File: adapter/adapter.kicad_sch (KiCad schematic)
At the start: 28 parts, among them J1 Serial, J10 Ribbon, J11 SPI user, J12 SPI user, J2 Serial, J3 RGB, J4 RGB, J5 Trackball, J6 Ribbon, J7 Trackball, J8 Ribbon, J9 Ribbon, SW1 USER, SW2 USER, U1 STM32F401 / STM32F411 Blackpi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, U2 STM32F401 / STM32F411 Blackpi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

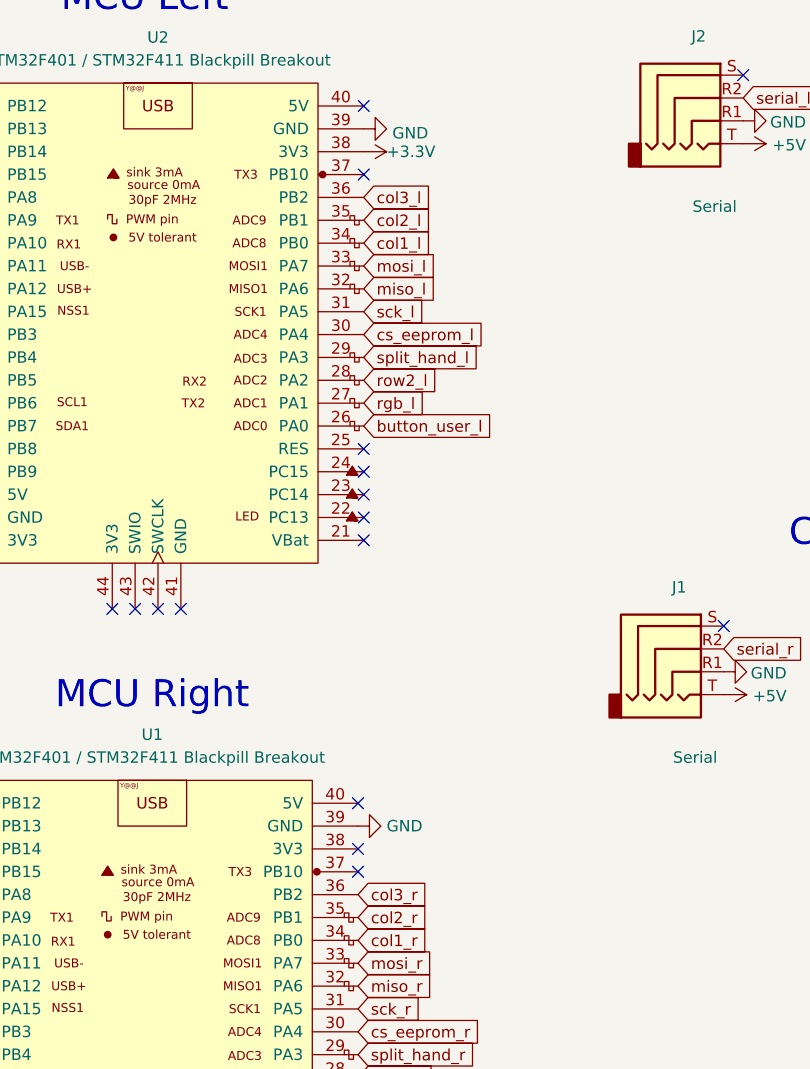
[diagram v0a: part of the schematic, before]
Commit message: Bugfix release 1.1
PB2 has a pulldown on the WeACT board to ensure BOOT1
is low during boot up. Otherwise jumping into the bootloader
is not ensured. So COL3 is moved from PB2 to PB10 as the pull
down prevents this pin from beeing used for matrix scanning.
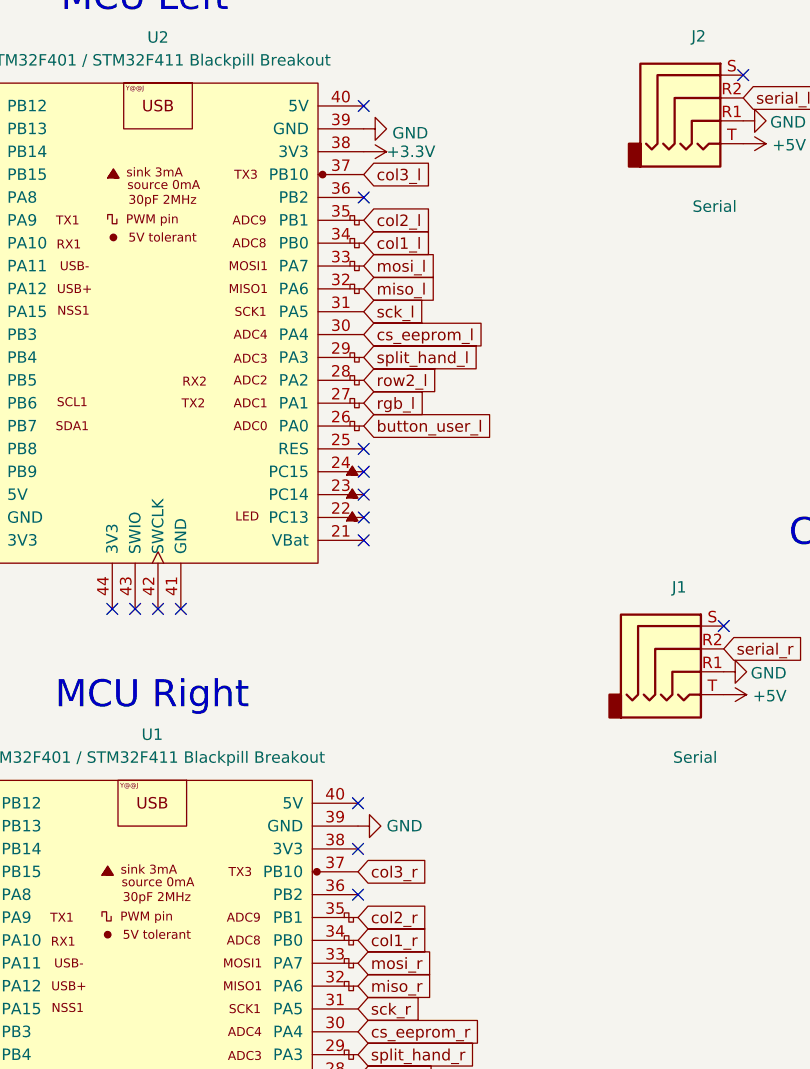
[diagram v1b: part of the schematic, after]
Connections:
- net col3_l: now also U2.37 (PB10); no longer U2.36 (PB2)
- net col3_r: now also U1.37 (PB10); no longer U1.36 (PB2)
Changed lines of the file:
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@@
   (no_connect (at 135.255 168.275))
   (no_connect (at 117.475 112.395))
-  (no_connect (at 163.195 120.015))
   (no_connect (at 118.11 34.925))
+  (no_connect (at 163.195 122.555))
   (no_connect (at 117.475 114.935))
   (no_connect (at 163.195 158.115))
@@
   (no_connect (at 205.994 31.496))
   (no_connect (at 163.83 34.925))
+  (no_connect (at 163.83 45.085))
   (no_connect (at 118.11 37.465))
-  (no_connect (at 163.83 42.545))
   (no_connect (at 163.195 153.035))
   (no_connect (at 118.11 52.705))
@@
     )
   )
-  (global_label "col3_r" (shape input) (at 163.195 122.555 0)
-    (effects (font (size 1.27 1.27)) (justify left))
-    (property "Intersheet References" "${INTERSHEET_REFS}" (id 0) (at 192.405 161.925 0)
+  (global_label "col3_r" (shape input) (at 163.195 120.015 0)
+    (effects (font (size 1.27 1.27)) (justify left))
+    (property "Intersheet References" "${INTERSHEET_REFS}" (id 0) (at 192.405 159.385 0)
       (effects (font (size 1.27 1.27)) hide)
     )
@@
     )
   )
-  (global_label "col3_l" (shape input) (at 163.83 45.085 0)
-    (effects (font (size 1.27 1.27)) (justify left))
-    (property "Intersheet References" "${INTERSHEET_REFS}" (id 0) (at 193.04 84.455 0)
-      (effects (font (size 1.27 1.27)) hide)
-    )
+  (global_label "col3_l" (shape input) (at 163.83 42.545 0)
+    (effects (font (size 1.27 1.27)) (justify left))
+    (property "Intersheet References" "${INTERSHEET_REFS}" (id 0) (at 193.04 81.915 0)
+      (effects (font (size 1.27 1.27)) hide)
+    )

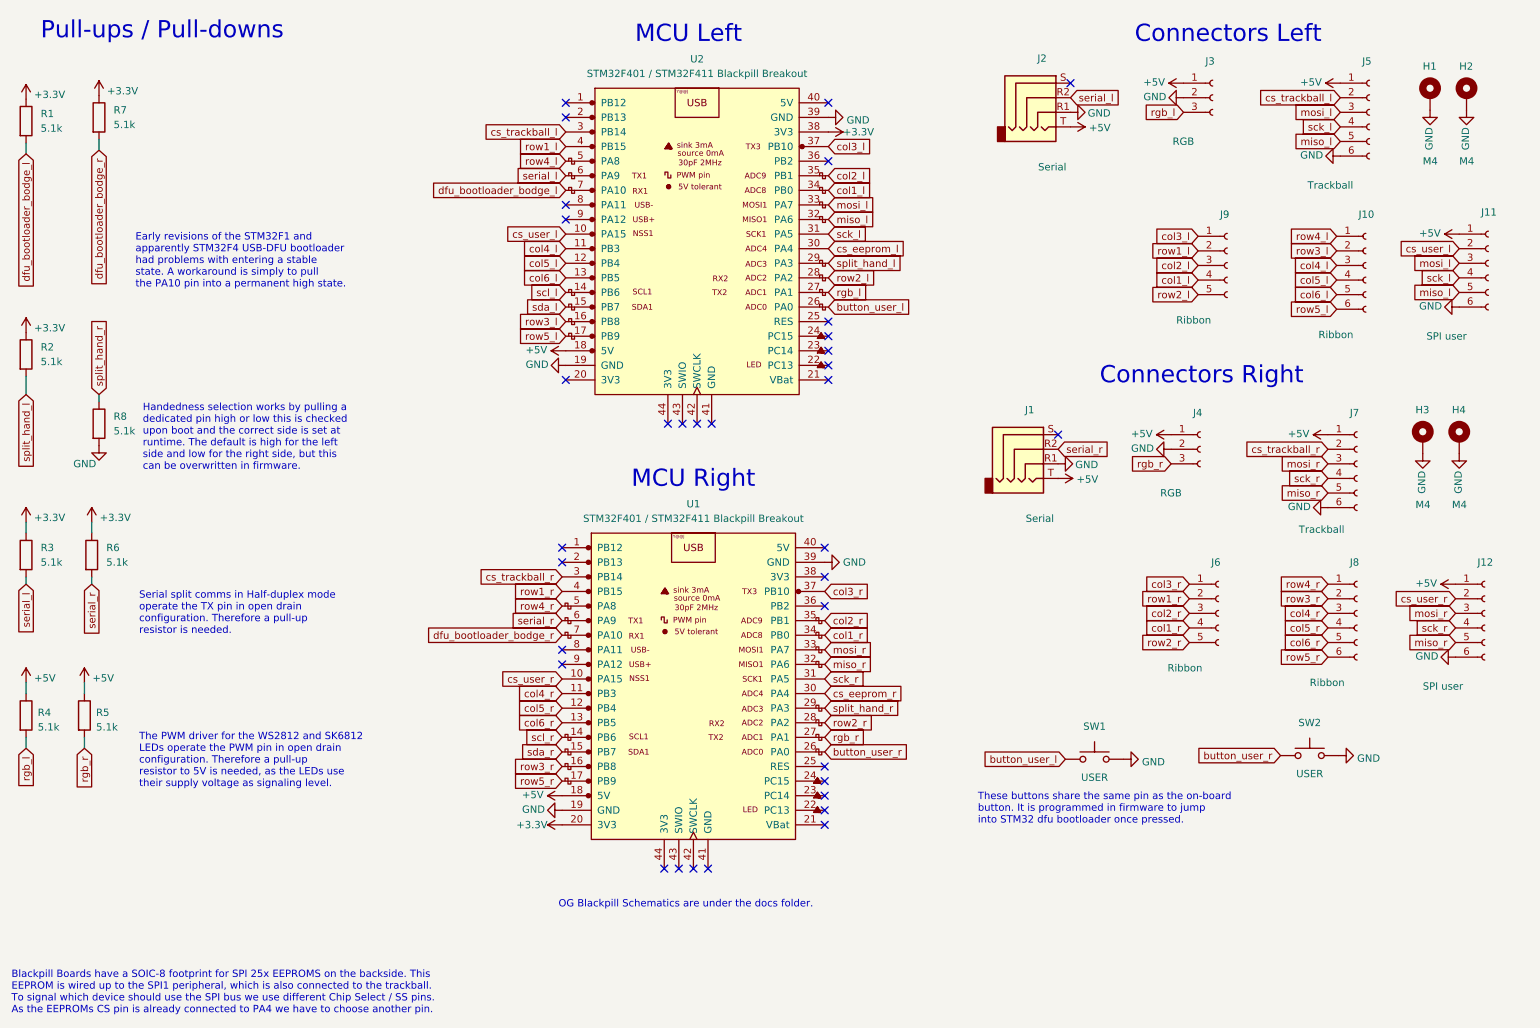
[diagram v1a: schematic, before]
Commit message: Remove SPI user, add breakouts for audio and row 6
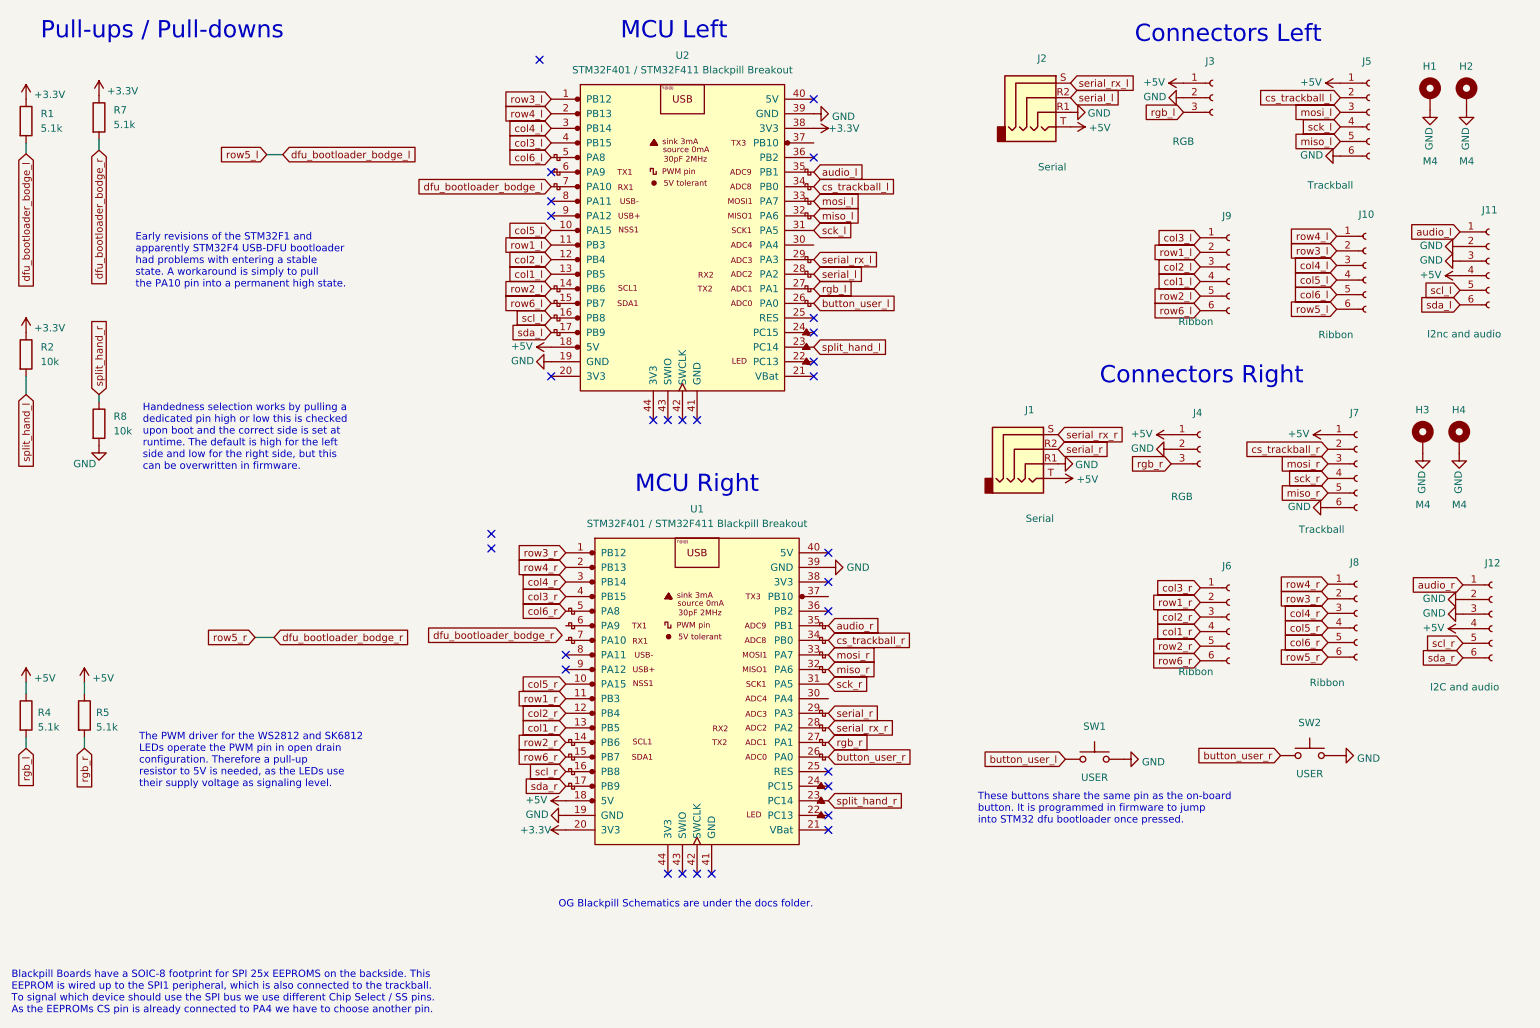
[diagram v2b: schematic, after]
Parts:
- removed R3, R6: 5.1k, Resistor_SMD:R_1206_3216Metric_Pad1.30x1.75mm_HandSolder, symbol Device:R
- J11: value SPI user -> I2nc and audio
- J12: value SPI user -> I2C and audio
- J6, J9: footprint Library:5_PinHeader -> Library:6_PinHeader; symbol Connector:Conn_01x05_Female -> Connector:Conn_01x06_Female
- R1, R4, R5, R7: footprint Resistor_SMD:R_1206_3216Metric_Pad1.30x1.75mm_HandSolder -> Resistor_SMD:R_0805_2012Metric_Pad1.20x1.40mm_HandSolder
- R2, R8: value 5.1k -> 10k; footprint Resistor_SMD:R_1206_3216Metric_Pad1.30x1.75mm_HandSolder -> Resistor_SMD:R_0805_2012Metric_Pad1.20x1.40mm_HandSolder
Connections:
- net +5V: now also J11.4 (Pin_4), J12.4 (Pin_4); no longer J11.1 (Pin_1), J12.1 (Pin_1)
- net GND: now also J11.2 (Pin_2), J11.3 (Pin_3), J12.2 (Pin_2), J12.3 (Pin_3); no longer J11.6 (Pin_6), J12.6 (Pin_6)
- net col1_l: now also U2.13 (PB5); no longer U2.34 (PB0)
- net col1_r: now also U1.13 (PB5); no longer U1.34 (PB0)
- net col2_l: now also U2.12 (PB4); no longer U2.35 (PB1)
- net col2_r: now also U1.12 (PB4); no longer U1.35 (PB1)
- net col3_l: now also U2.4 (PB15); no longer U2.37 (PB10)
- net col3_r: now also U1.4 (PB15); no longer U1.37 (PB10)
- net col4_l: now also U2.3 (PB14); no longer U2.11 (PB3)
- net col4_r: now also U1.3 (PB14); no longer U1.11 (PB3)
- net col5_l: now also U2.10 (PA15); no longer U2.12 (PB4)
- net col5_r: now also U1.10 (PA15); no longer U1.12 (PB4)
- net col6_l: now also U2.5 (PA8); no longer U2.13 (PB5)
- net col6_r: now also U1.5 (PA8); no longer U1.13 (PB5)
- net cs_trackball_l: now also U2.34 (PB0); no longer U2.3 (PB14)
- net cs_trackball_r: now also U1.34 (PB0); no longer U1.3 (PB14)
- net dfu_bootloader_bodge_l: now also J10.6 (Pin_6)
- net dfu_bootloader_bodge_r: now also J8.6 (Pin_6); no longer U1.7 (PA10)
- net miso_l: no longer J11.5 (Pin_5)
- net miso_r: no longer J12.5 (Pin_5)
- net mosi_l: no longer J11.3 (Pin_3)
- net mosi_r: no longer J12.3 (Pin_3)
- net row1_l: now also U2.11 (PB3); no longer U2.4 (PB15)
- net row1_r: now also U1.11 (PB3); no longer U1.4 (PB15)
- net row2_l: now also U2.14 (PB6); no longer U2.28 (PA2)
- net row2_r: now also U1.14 (PB6); no longer U1.28 (PA2)
- net row3_l: now also U2.1 (PB12); no longer U2.16 (PB8)
- net row3_r: now also U1.1 (PB12); no longer U1.16 (PB8)
- net row4_l: now also U2.2 (PB13); no longer U2.5 (PA8)
- net row4_r: now also U1.2 (PB13); no longer U1.5 (PA8)
- net sck_l: no longer J11.4 (Pin_4)
- net sck_r: no longer J12.4 (Pin_4)
- net scl_l: now also J11.5 (Pin_5), U2.16 (PB8); no longer U2.14 (PB6)
- net scl_r: now also J12.5 (Pin_5), U1.16 (PB8); no longer U1.14 (PB6)
- net sda_l: now also J11.6 (Pin_6), U2.17 (PB9); no longer U2.15 (PB7)
- net sda_r: now also J12.6 (Pin_6), U1.17 (PB9); no longer U1.15 (PB7)
- net serial_l: now also U2.28 (PA2); no longer U2.6 (PA9)
- net serial_r: now also U1.29 (PA3); no longer U1.6 (PA9)
- net split_hand_l: now also U2.23 (PC14); no longer U2.29 (PA3)
- net split_hand_r: now also U1.23 (PC14); no longer U1.29 (PA3)
- net serial_rx_r: now reaches J1.S
- net serial_rx_r: now also U1.28 (PA2)
- net serial_rx_l: now reaches J2.S
- net serial_rx_l: now also U2.29 (PA3)
- net cs_eeprom_l: no longer names the net of U2.30 (PA4)
- net cs_eeprom_r: no longer names the net of U1.30 (PA4)
- removed net cs_user_l: J11.2 (Pin_2), U2.10 (PA15)
- removed net cs_user_r: J12.2 (Pin_2), U1.10 (PA15)
- removed net row5_l: J10.6 (Pin_6), U2.17 (PB9)
- removed net row5_r: J8.6 (Pin_6), U1.17 (PB9)
- new net audio_l: J11.1 (Pin_1), U2.35 (PB1)
- new net audio_r: J12.1 (Pin_1), U1.35 (PB1)
- new net row6_l: J9.6 (Pin_6), U2.15 (PB7)
- new net row6_r: J6.6 (Pin_6), U1.15 (PB7)
- no-connect marks 34 -> 30
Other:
- note removed: "Serial split comms in Half-duplex mode operate the TX pin in open drain configuration. Therefore a pull-up resistor is needed."
- moved on the sheet: J12, U1, U2
